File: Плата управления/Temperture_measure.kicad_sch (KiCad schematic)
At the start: 14 parts, among them U3 LMV324

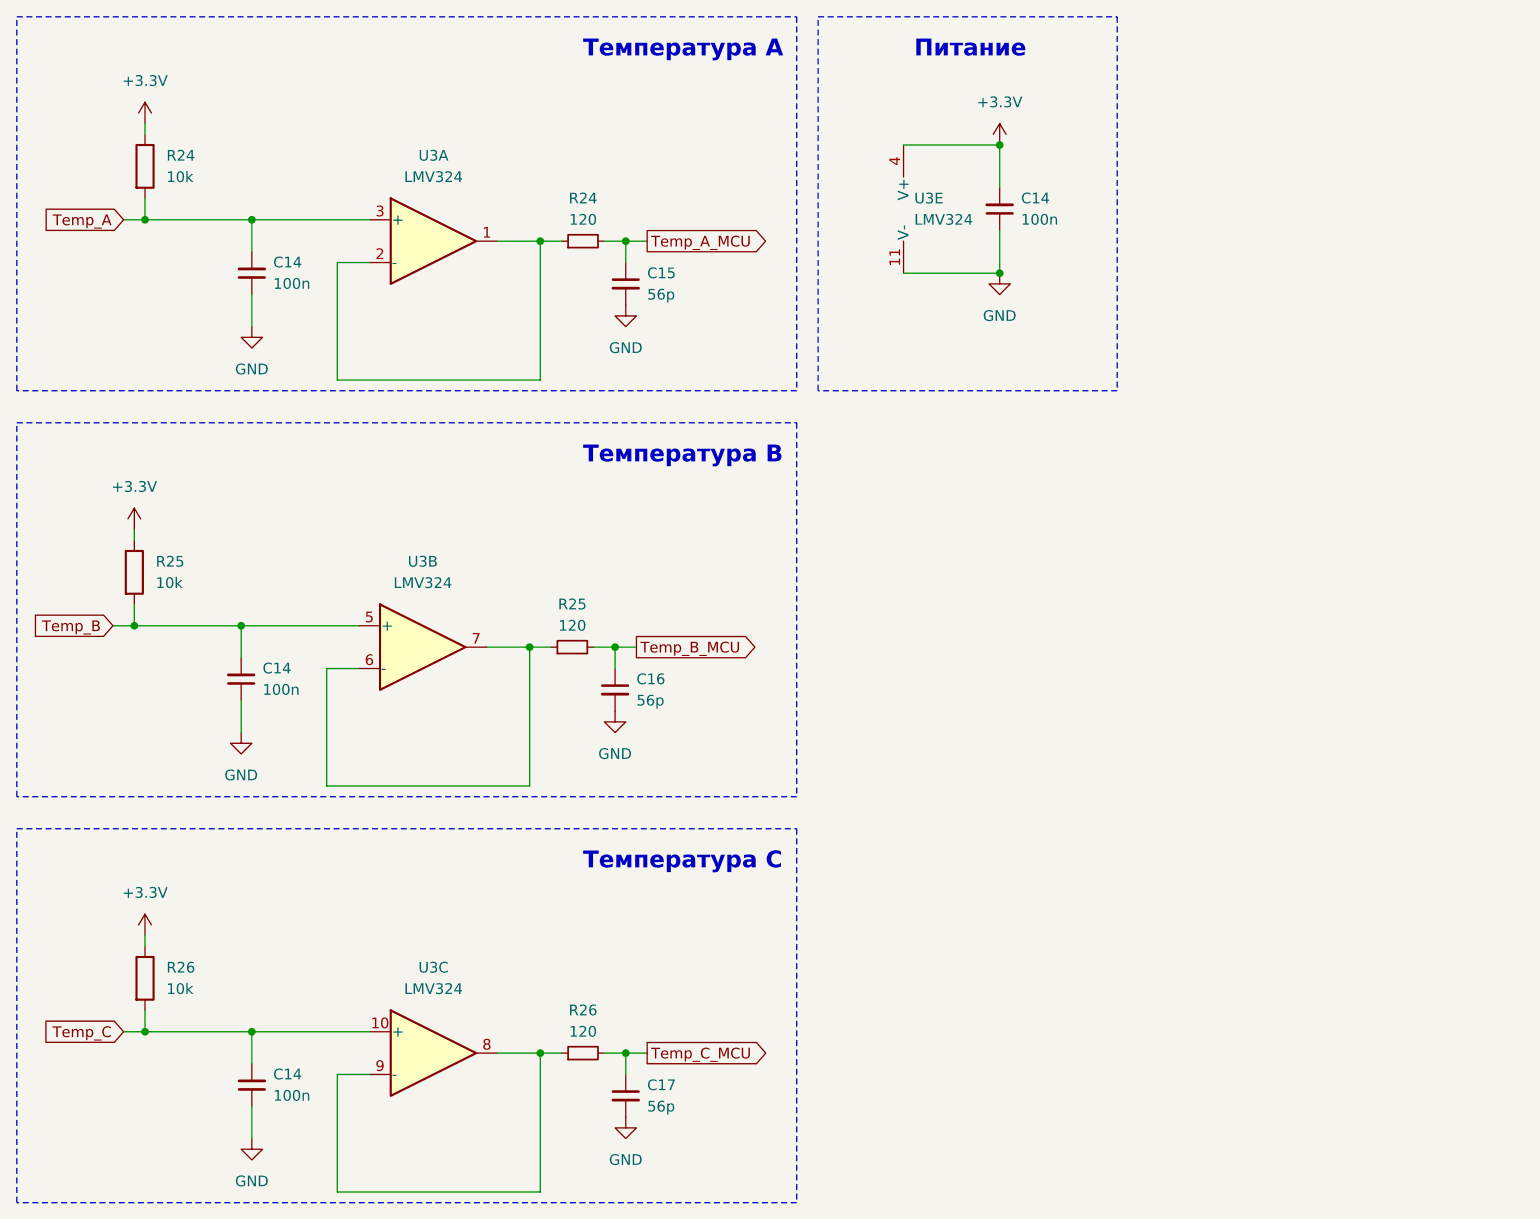
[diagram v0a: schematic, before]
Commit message: Новый контур платы
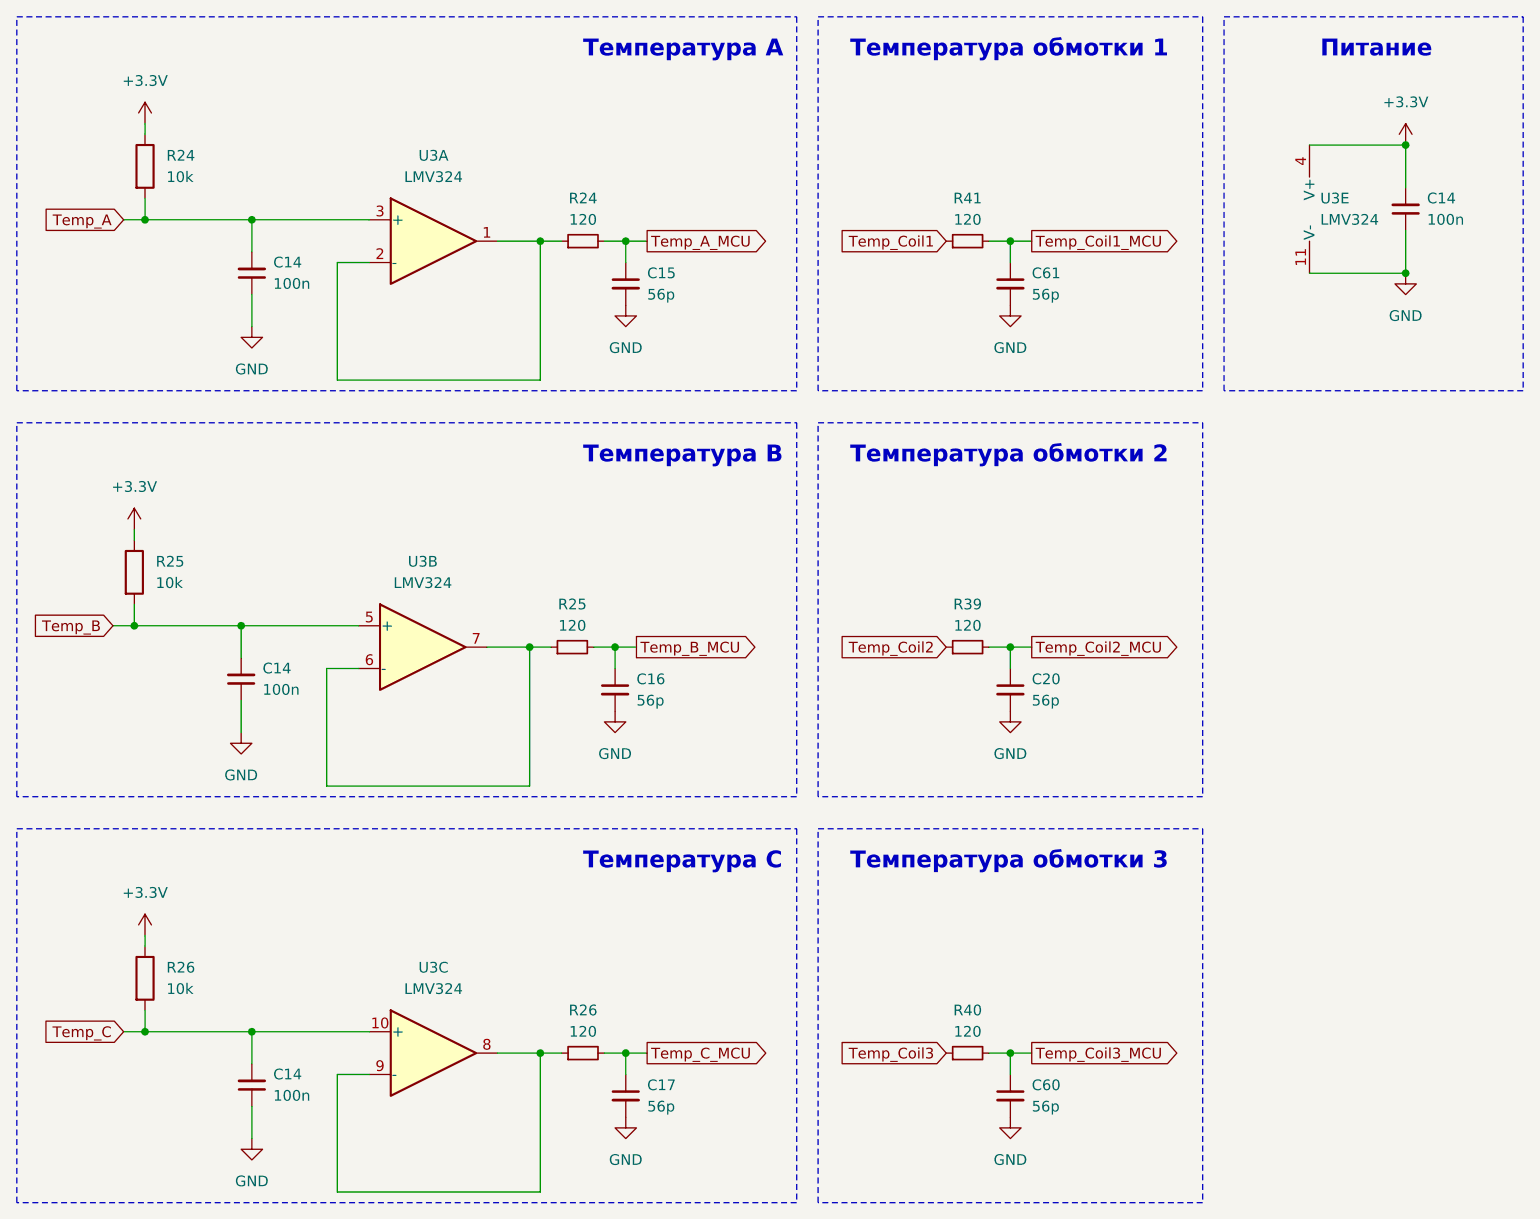
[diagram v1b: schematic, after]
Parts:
- added C20, C60, C61: 56p, Capacitor_SMD:C_0603_1608Metric_Pad1.08x0.95mm_HandSolder, symbol Device:C_Small
- added R39, R40, R41: 120, Resistor_SMD:R_0603_1608Metric_Pad0.98x0.95mm_HandSolder, symbol Device:R_Small
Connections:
- net GND: now also C20.2, C60.2, C61.2
- new net Temp_Coil1: R41.1
- new net Temp_Coil1_MCU: C61.1, R41.2
- new net Temp_Coil2: R39.1
- new net Temp_Coil2_MCU: C20.1, R39.2
- new net Temp_Coil3: R40.1
- new net Temp_Coil3_MCU: C60.1, R40.2
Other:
- note added: "Температура обмотки 1"
- note added: "Температура обмотки 2"
- note added: "Температура обмотки 3"
- moved on the sheet: C14, U3E
